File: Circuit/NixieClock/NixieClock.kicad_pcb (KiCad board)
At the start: 2 copper layers, 26 x 61 mm, 14 parts, among them J1 Conn_01x10, Q1 MMBTA42, U1 74141N, U2 74AHC595

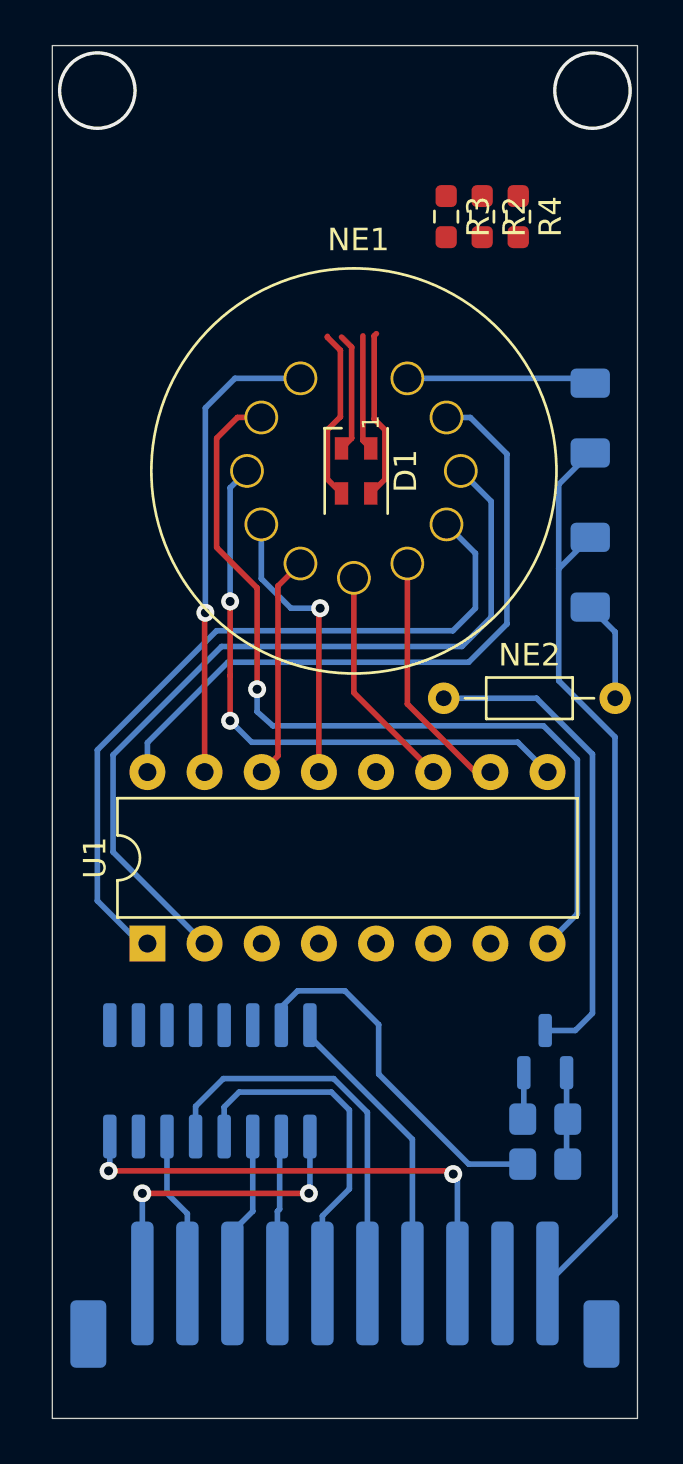
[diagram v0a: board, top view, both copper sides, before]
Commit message: Complete Route
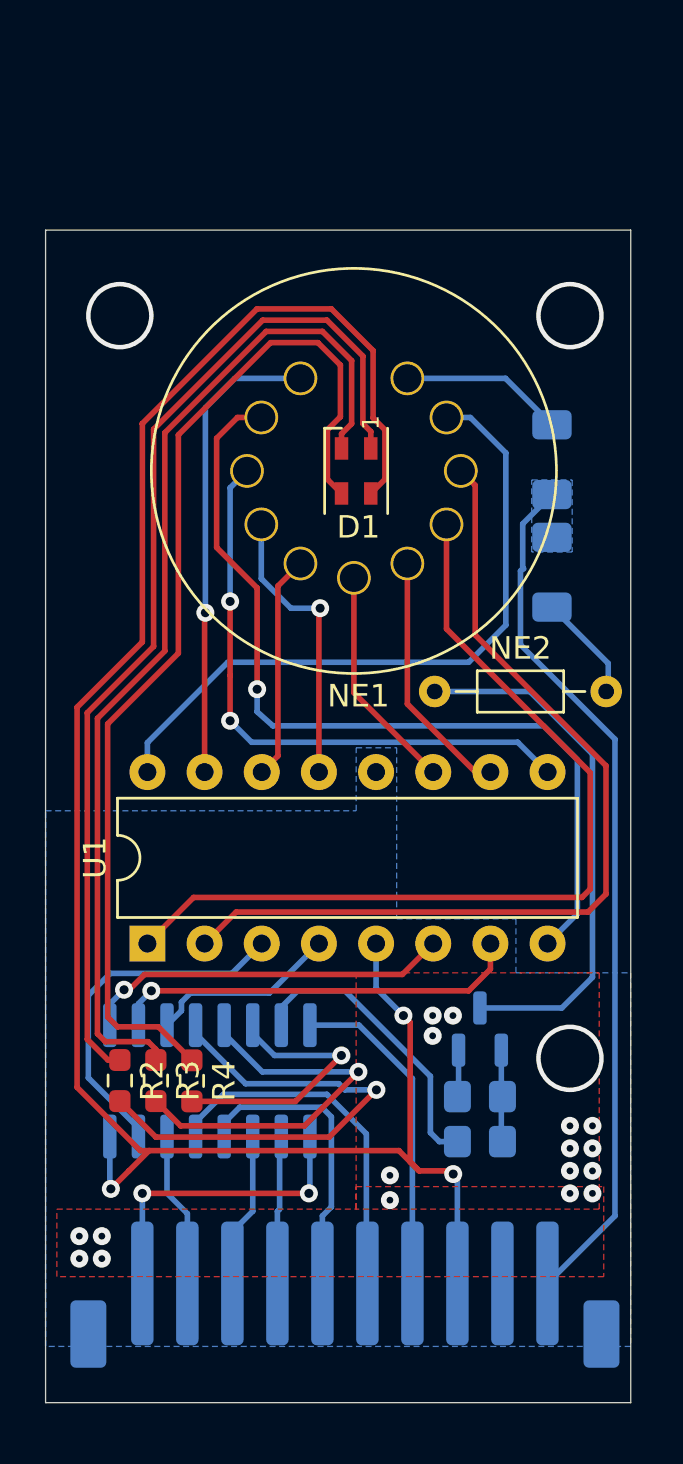
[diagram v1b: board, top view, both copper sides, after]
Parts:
- moved R2 41.6 mm to (23.0, 66.0)
- moved R4 41.0 mm to (26.2, 66.0)
- moved R3 40.5 mm to (24.6, 66.0)
- moved Q1 3.07 mm to (39.0, 63.7)
- moved R5 3.07 mm to (39.0, 68.7)
- moved R6 3.07 mm to (39.0, 66.7)
- moved R1 2.51 mm to (42.2, 38.4)
- moved R7 1.70 mm to (42.2, 43.4)
- moved NE2 0.50 mm to (37.0, 48.7)
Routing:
- net +5V: track 29.5 -> 89.5 mm, vias 2 -> 3
- net Net-(D1-Pad1): track 5.14 -> 46.4 mm
- net Net-(D1-Pad2): track 5.32 -> 46.1 mm
- net Net-(D1-Pad3): track 7.72 -> 47.2 mm
- net Net-(R2-Pad2): track 0.00 -> 22.4 mm, vias 0 -> 1
- net Net-(U1-Pad7): track 0.00 -> 18.4 mm, vias 0 -> 1
- net Net-(R3-Pad2): track 0.00 -> 17.5 mm, vias 0 -> 1
- net Net-(U1-Pad6): track 0.00 -> 16.9 mm, vias 0 -> 1
- net Net-(U1-Pad3): track 0.00 -> 15.9 mm
- net Net-(R4-Pad2): track 0.00 -> 12.2 mm, vias 0 -> 1
- net Net-(U1-Pad4): track 0.00 -> 8.47 mm
- net Net-(NE1-Pad8): track 33.4 -> 39.5 mm
- net Net-(NE1-Pad9): track 36.5 -> 40.2 mm
- net Net-(R5-Pad1): track 16.3 -> 13.2 mm
- net /HV_DC: track 41.7 -> 38.6 mm
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- added copper zone on B.Cu, net /HV_DC
- added copper zone on B.Cu, net GND
- added copper zone on F.Cu, net GND
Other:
- board size 26 x 61 mm -> 26 x 52.1 mm
